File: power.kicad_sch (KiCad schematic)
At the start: 27 parts, among them U100 B0505XT-1WR3, U22 TLV76733DRVx, U6 LMR14006

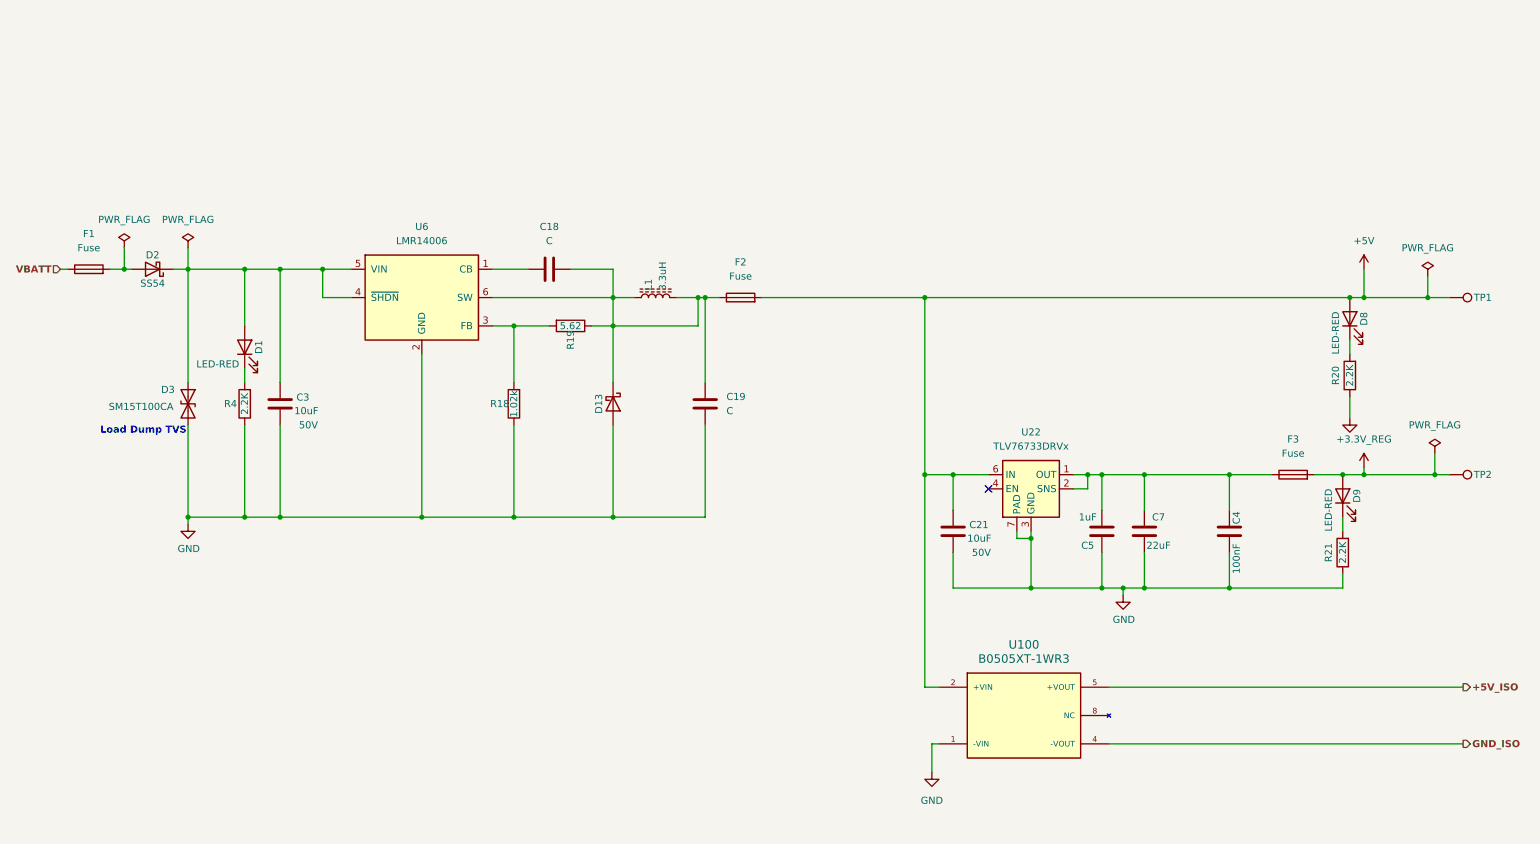
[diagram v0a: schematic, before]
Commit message: SENT TO jlcpcb
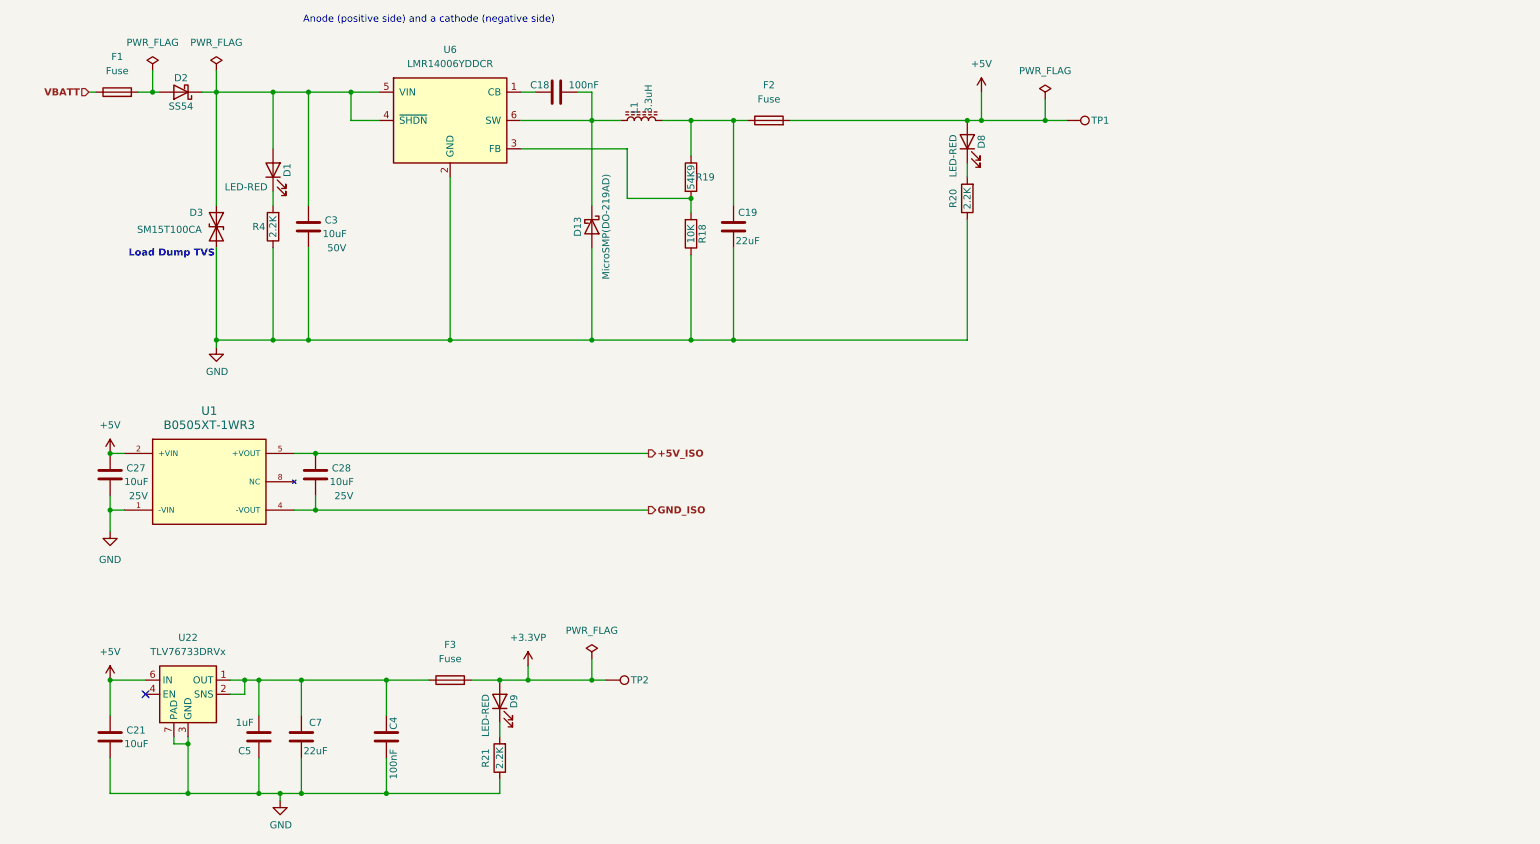
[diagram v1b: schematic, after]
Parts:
- removed U100: B0505XT-1WR3, dnt:0505_Isolated_SMD, symbol dnt:0505_Isolated_SMD
- added C27, C28: 10uF, Capacitor_SMD:C_0603_1608Metric, symbol Device:C
- added U1: B0505XT-1WR3, dnt:0505_Isolated_SMD, symbol dnt:0505_Isolated_SMD
- C18: value C -> 100nF; footprint Capacitor_SMD:C_0805_2012Metric -> Capacitor_SMD:C_0603_1608Metric; LCSC (none) -> C14663; Manufacturer (none) -> YAGEO; Part Number (none) -> CC0603KRX7R9BB104
- C19: value C -> 22uF; LCSC (none) -> C45783; Voltage (none) -> 25V
- C21: footprint Capacitor_SMD:C_0805_2012Metric -> Capacitor_SMD:C_0603_1608Metric; LCSC C440198 -> C96446; PN GRM21BR61H106KE43L -> (none); Voltage 50V -> (none)
- C3: Vendor (none) -> Murata Electronics
- D1, D8, D9: JLCPCB Rotation Offset 180 -> 0
- D13: value ~ -> MicroSMP(DO-219AD)
- D2: JLCPCB Rotation Offset 180 -> 0; Silkscreen X -> (none)
- R18: value 1.02k -> 10K; LCSC C858881 -> C25804; Manufacturer YAGEO -> StackPole; Part # RC0603DR-071K02L -> RMCF0603JT10K0; VEND (none) -> DIGI; VEND# (none) -> RMCF0603JT10K0CT-ND
- R19: value 5.62 -> 54K9; LCSC C855916 -> C185321; Part # AT0603BRD075K62L -> RC0603FR-0754K9L; Silkscreen (none) -> Hmm
- U6: value LMR14006 -> LMR14006YDDCR; JLCPCB Rotation Offset (none) -> -90; LCSC (none) -> C477919; Order (none) -> https://jlcpcb.com/partdetail/TexasInstruments-LMR14006YDDC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; Package (none) -> TSOT-23-6
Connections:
- net +5V: now also C27.1, U1.2 (+VIN)
- net +5V_ISO: now also C28.1, U1.5 (+VOUT)
- net GND: now also C27.2, U1.1 (-VIN)
- net GND_ISO: now also C28.2, U1.4 (-VOUT)
- net at C18.2, D13.1 (K), L1.1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: no longer C19.1, F2.1, L1.2, R19.1
- net +3.3V_REG renamed +3.3VP
- new net: C19.1, F2.1, L1.2, R19.1
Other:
- note added: "Anode (positive side) and a cathode (negative side)"
- moved on the sheet: C21, C3, C4, C5, C7, D1, D13, D2, D3, D8, D9, F1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
